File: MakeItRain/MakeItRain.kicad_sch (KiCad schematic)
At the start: 15 parts, among them J1 Conn_02x14_Odd_Even, J2 Conn_02x19_Odd_Even, J3 Conn_01x19, U1 MCP23008-xP

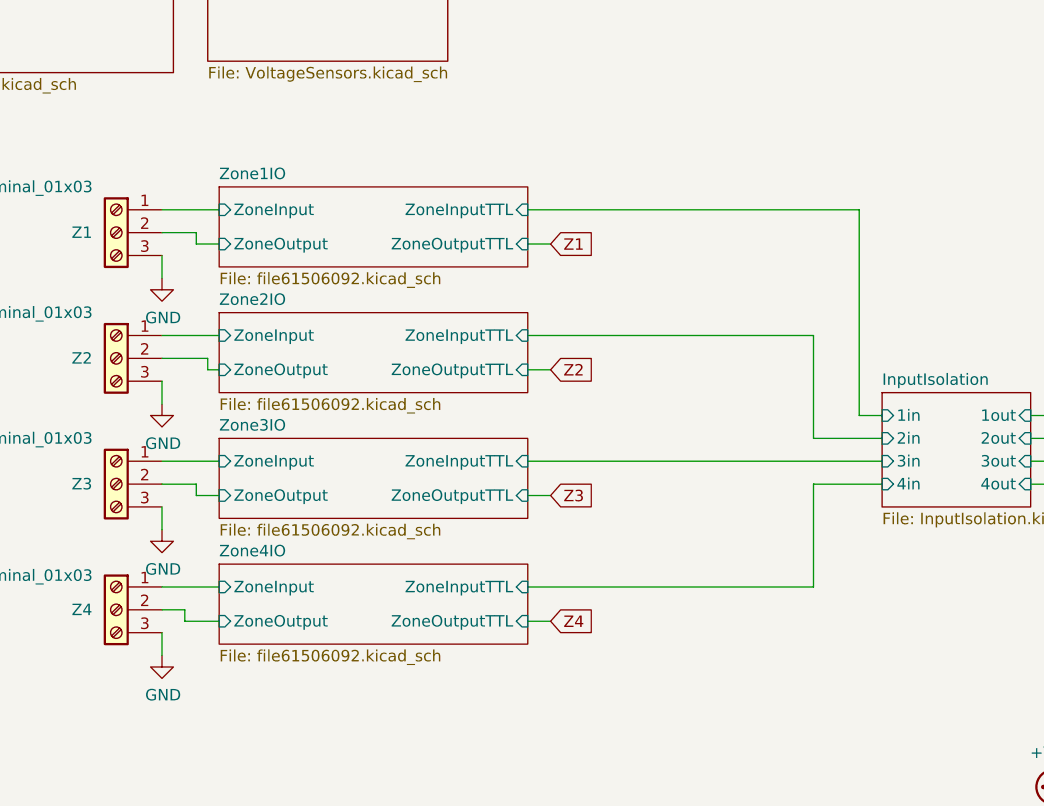
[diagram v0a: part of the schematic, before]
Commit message: imput redesign
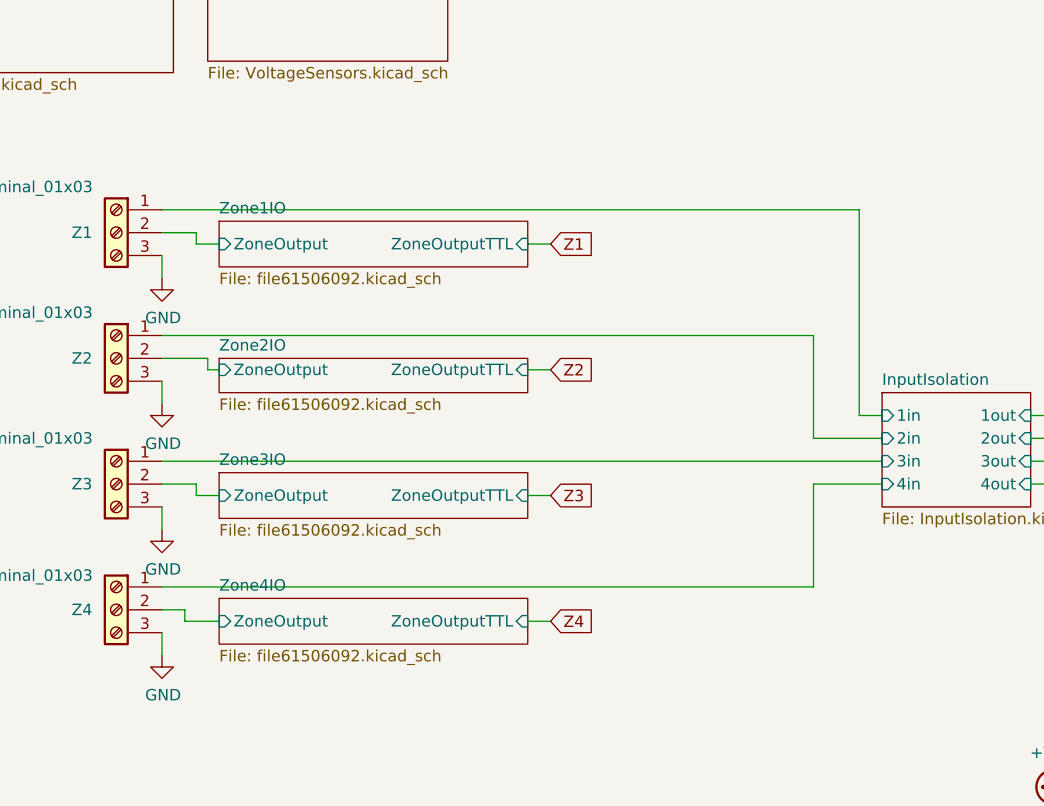
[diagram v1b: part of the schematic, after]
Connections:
- net Zone1IO/ZoneInput is gone; now on net InputIsolation/1in: Z1.1 (Pin_1)
- net Zone2IO/ZoneInput is gone; now on net InputIsolation/2in: Z2.1 (Pin_1)
- net Zone3IO/ZoneInput is gone; now on net InputIsolation/3in: Z3.1 (Pin_1)
- net Zone4IO/ZoneInput is gone; now on net InputIsolation/4in: Z4.1 (Pin_1)
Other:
- sheet Zone1IO ports: added none; removed ZoneInput, ZoneInputTTL
- sheet Zone2IO ports: added none; removed ZoneInput, ZoneInputTTL
- sheet Zone3IO ports: added none; removed ZoneInput, ZoneInputTTL
- sheet Zone4IO ports: added none; removed ZoneInput, ZoneInputTTL
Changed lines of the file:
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@@
-    (stroke (width 0) (type default))
-  )
-  (wire (pts (xy 44.45 88.9) (xy 50.8 88.9))
     (stroke (width 0) (type default))
   )
@@
     (stroke (width 0) (type default))
   )
-  (wire (pts (xy 85.09 46.99) (xy 121.92 46.99))
-    (stroke (width 0) (type default))
-  )
   (wire (pts (xy 233.68 107.95) (xy 220.98 107.95))
     (stroke (width 0) (type default))
@@
     (stroke (width 0) (type default))
   )
-  (wire (pts (xy 85.09 74.93) (xy 124.46 74.93))
-    (stroke (width 0) (type default))
-  )
   (wire (pts (xy 157.48 153.67) (xy 173.99 153.67))
     (stroke (width 0) (type default))
@@
     (stroke (width 0) (type default))
   )
-  (wire (pts (xy 116.84 88.9) (xy 85.09 88.9))
+  (wire (pts (xy 44.45 88.9) (xy 116.84 88.9))
     (stroke (width 0) (type default))
   )
@@
     (stroke (width 0) (type default))
   )
+  (wire (pts (xy 44.45 46.99) (xy 121.92 46.99))
+    (stroke (width 0) (type default))
+  )
   (wire (pts (xy 246.38 125.73) (xy 261.62 125.73))
     (stroke (width 0) (type default))
@@
     (stroke (width 0) (type default))
   )
-  (wire (pts (xy 44.45 46.99) (xy 50.8 46.99))
-    (stroke (width 0) (type default))
-  )
   (wire (pts (xy 142.24 151.13) (xy 144.78 151.13))
     (stroke (width 0) (type default))
@@
     (stroke (width 0) (type default))
   )
-  (wire (pts (xy 50.8 60.96) (xy 44.45 60.96))
+  (wire (pts (xy 44.45 60.96) (xy 116.84 60.96))
     (stroke (width 0) (type default))
   )
@@
     (stroke (width 0) (type default))
   )
-  (wire (pts (xy 44.45 74.93) (xy 50.8 74.93))
+  (wire (pts (xy 44.45 74.93) (xy 124.46 74.93))
     (stroke (width 0) (type default))
   )
@@
   )
   (wire (pts (xy 213.36 107.95) (xy 220.98 107.95))
-    (stroke (width 0) (type default))
-  )
-  (wire (pts (xy 116.84 60.96) (xy 85.09 60.96))
     (stroke (width 0) (type default))
   )
@@
     )
   )
-  (sheet (at 50.8 44.45) (size 34.29 8.89) (fields_autoplaced)
+  (sheet (at 50.8 48.26) (size 34.29 5.08) (fields_autoplaced)
     (stroke (width 0) (type solid))
     (fill (color 0 0 0 0.0000))
-    (property "Sheetname" "Zone1IO" (at 50.8 43.7384 0)
+    (property "Sheetname" "Zone1IO" (at 50.8 47.5484 0)
       (effects (font (size 1.27 1.27)) (justify left bottom))
     )
@@
       (effects (font (size 1.27 1.27)) (justify left top))
     )
-    (pin "ZoneInput" input (at 50.8 46.99 180)
-      (effects (font (size 1.27 1.27)) (justify left))
-    )
-    (pin "ZoneInputTTL" input (at 85.09 46.99 0)
-      (effects (font (size 1.27 1.27)) (justify right))
-    )
     (pin "ZoneOutputTTL" input (at 85.09 50.8 0)
       (effects (font (size 1.27 1.27)) (justify right))
@@
     )
   )
-  (sheet (at 50.8 58.42) (size 34.29 8.89) (fields_autoplaced)
+  (sheet (at 50.8 63.5) (size 34.29 3.81) (fields_autoplaced)
     (stroke (width 0) (type solid))
     (fill (color 0 0 0 0.0000))
-    (property "Sheetname" "Zone2IO" (at 50.8 57.7084 0)
+    (property "Sheetname" "Zone2IO" (at 50.8 62.7884 0)
       (effects (font (size 1.27 1.27)) (justify left bottom))
     )
@@
       (effects (font (size 1.27 1.27)) (justify left top))
     )
-    (pin "ZoneInput" input (at 50.8 60.96 180)
-      (effects (font (size 1.27 1.27)) (justify left))
-    )
-    (pin "ZoneInputTTL" input (at 85.09 60.96 0)
-      (effects (font (size 1.27 1.27)) (justify right))
-    )
     (pin "ZoneOutputTTL" input (at 85.09 64.77 0)
       (effects (font (size 1.27 1.27)) (justify right))
@@
     )
   )
-  (sheet (at 50.8 72.39) (size 34.29 8.89) (fields_autoplaced)
+  (sheet (at 50.8 76.2) (size 34.29 5.08) (fields_autoplaced)
     (stroke (width 0) (type solid))
     (fill (color 0 0 0 0.0000))
-    (property "Sheetname" "Zone3IO" (at 50.8 71.6784 0)
+    (property "Sheetname" "Zone3IO" (at 50.8 75.4884 0)
       (effects (font (size 1.27 1.27)) (justify left bottom))
     )
@@
       (effects (font (size 1.27 1.27)) (justify left top))
     )
-    (pin "ZoneInput" input (at 50.8 74.93 180)
-      (effects (font (size 1.27 1.27)) (justify left))
-    )
-    (pin "ZoneInputTTL" input (at 85.09 74.93 0)
-      (effects (font (size 1.27 1.27)) (justify right))
-    )
     (pin "ZoneOutputTTL" input (at 85.09 78.74 0)
       (effects (font (size 1.27 1.27)) (justify right))
@@
     )
   )
-  (sheet (at 50.8 86.36) (size 34.29 8.89) (fields_autoplaced)
+  (sheet (at 50.8 90.17) (size 34.29 5.08) (fields_autoplaced)
     (stroke (width 0) (type solid))
     (fill (color 0 0 0 0.0000))
-    (property "Sheetname" "Zone4IO" (at 50.8 85.6484 0)
+    (property "Sheetname" "Zone4IO" (at 50.8 89.4584 0)
       (effects (font (size 1.27 1.27)) (justify left bottom))
     )
@@
       (effects (font (size 1.27 1.27)) (justify left top))
     )
-    (pin "ZoneInput" input (at 50.8 88.9 180)
-      (effects (font (size 1.27 1.27)) (justify left))
-    )
-    (pin "ZoneInputTTL" input (at 85.09 88.9 0)
-      (effects (font (size 1.27 1.27)) (justify right))
-    )
     (pin "ZoneOutputTTL" input (at 85.09 92.71 0)
